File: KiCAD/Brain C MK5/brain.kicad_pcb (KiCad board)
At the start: 2 copper layers, 143 x 44.8 mm, 20 parts, among them J1 USB_B, J10 Conn_01x10, J11 Conn_01x10, J2 Conn_01x06, J3 Conn_01x10, J4 Conn_01x06, J5 Conn_01x06, J6 Conn_01x06, J7 Conn_01x04, J8 Conn_01x04, J9 Conn_01x10

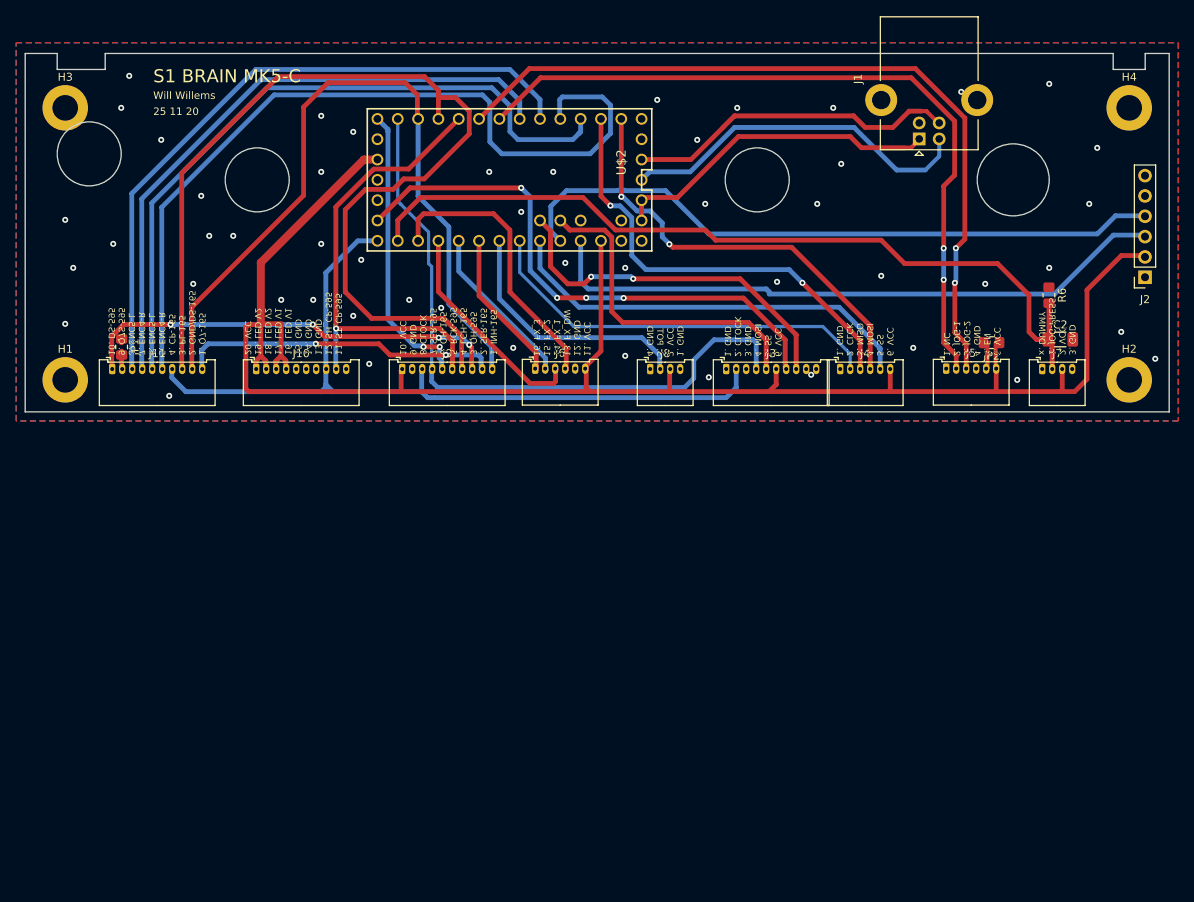
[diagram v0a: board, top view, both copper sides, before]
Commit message: add nect-gen KiCAD files
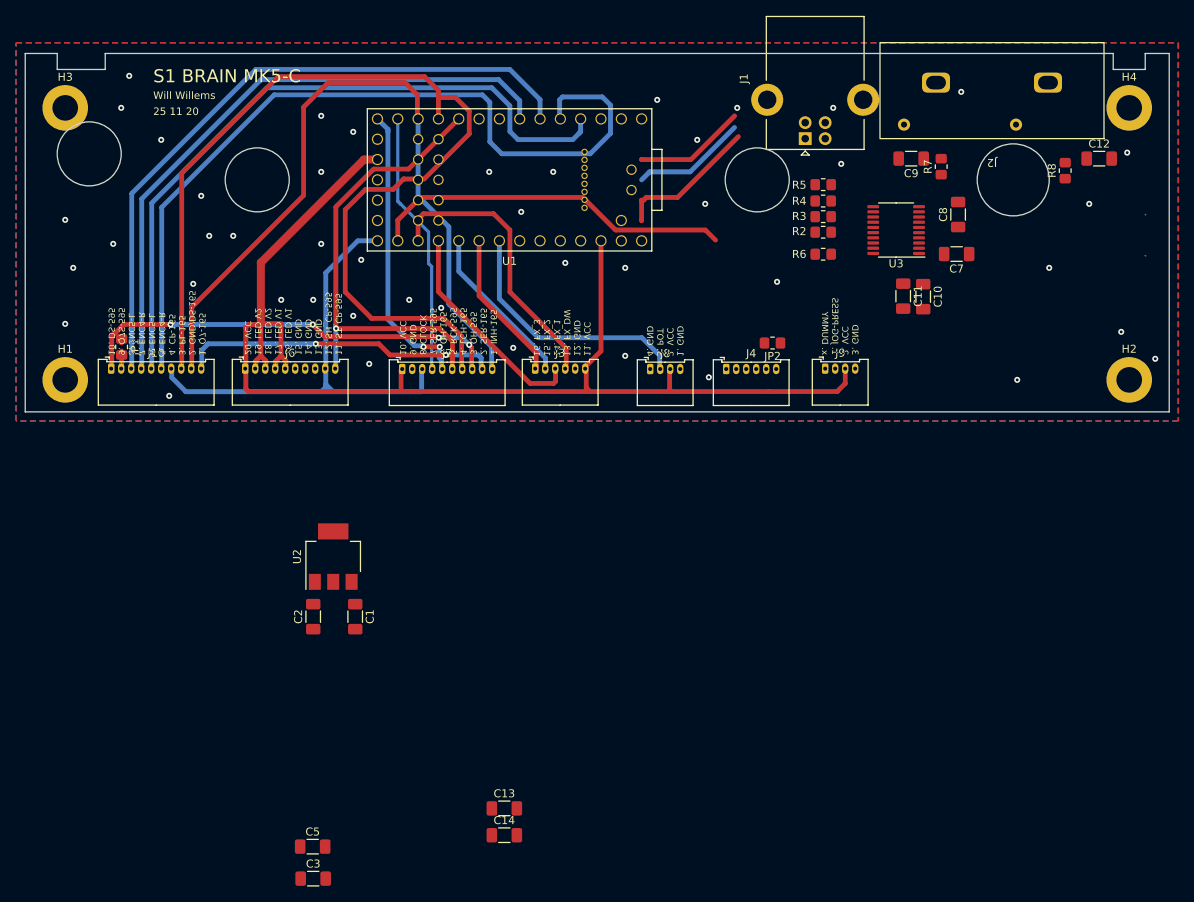
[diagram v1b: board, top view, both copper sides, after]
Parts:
- removed J11: Conn_01x10, Connector_Molex:Molex_PicoBlade_53048-1010_1x10_P1.25mm_Horizontal
- removed J5: Conn_01x06, Connector_Molex:Molex_PicoBlade_53048-0610_1x06_P1.25mm_Horizontal
- removed U$2: TEENSY_LC_ALL_PINS, brain:TEENSY_3.0-3.2&LC_ALL_PINS
- added C1: 100nF, Capacitor_SMD:C_1206_3216Metric_Pad1.33x1.80mm_HandSolder, F.Cu at (118.2, 153.0)
- added C10: 100nF, Capacitor_SMD:C_1206_3216Metric_Pad1.33x1.80mm_HandSolder, F.Cu at (189.2, 113.0)
- added C11: 10uF, Capacitor_SMD:C_1206_3216Metric_Pad1.33x1.80mm_HandSolder, F.Cu at (186.8, 112.9)
- added C12: 2.2nF, Capacitor_SMD:C_1206_3216Metric_Pad1.33x1.80mm_HandSolder, F.Cu at (211.2, 95.8)
- added C13: 100nF, Capacitor_SMD:C_1206_3216Metric_Pad1.33x1.80mm_HandSolder, F.Cu at (136.9, 177.0)
- added C14: 10uF, Capacitor_SMD:C_1206_3216Metric_Pad1.33x1.80mm_HandSolder, F.Cu at (136.9, 180.3)
- added C3: 100nF, Capacitor_SMD:C_1206_3216Metric_Pad1.33x1.80mm_HandSolder, F.Cu at (113.0, 185.8)
- added C5: 10uF, Capacitor_SMD:C_1206_3216Metric_Pad1.33x1.80mm_HandSolder, F.Cu at (112.9, 181.8)
- added C7: 2.2uF, Capacitor_SMD:C_1206_3216Metric_Pad1.33x1.80mm_HandSolder, F.Cu at (193.4, 107.7)
- added C8: 2.2uF, Capacitor_SMD:C_1206_3216Metric_Pad1.33x1.80mm_HandSolder, F.Cu at (193.6, 102.7)
- added C9: 2.2nF, Capacitor_SMD:C_1206_3216Metric_Pad1.33x1.80mm_HandSolder, F.Cu at (187.8, 95.8)
- added R2: 22, Resistor_SMD:R_0805_2012Metric_Pad1.20x1.40mm_HandSolder, F.Cu at (176.8, 105.0)
- added R3: 22, Resistor_SMD:R_0805_2012Metric_Pad1.20x1.40mm_HandSolder, F.Cu at (176.8, 103.0)
- added R4: 22, Resistor_SMD:R_0805_2012Metric_Pad1.20x1.40mm_HandSolder, F.Cu at (176.8, 101.0)
- added R5: 22, Resistor_SMD:R_0805_2012Metric_Pad1.20x1.40mm_HandSolder, F.Cu at (176.8, 99.0)
- added R7: 470, Resistor_SMD:R_0805_2012Metric_Pad1.20x1.40mm_HandSolder, F.Cu at (191.5, 96.8)
- added R8: 470, Resistor_SMD:R_0805_2012Metric_Pad1.20x1.40mm_HandSolder, F.Cu at (207.0, 97.2)
- added U1: Teensy4.0, Teensy:Teensy40_SMT, F.Cu at (137.5, 98.4)
- added U2: LD1117S33TR_SOT223, Package_TO_SOT_SMD:SOT-223-3_TabPin2, F.Cu at (115.5, 145.5)
- added U3: PCM5102, Package_SO:TSSOP-20_4.4x6.5mm_P0.65mm, F.Cu at (185.9, 104.7)
- C2: value 1u -> 10uF
- J2: value Conn_01x06 -> Conn_Coaxial_x2_Isolated; footprint Connector_PinSocket_2.54mm:PinSocket_1x06_P2.54mm_Vertical -> Audio:RCA_double
- J3: value Conn_01x10 -> Conn_01x06; footprint Connector_Molex:Molex_PicoBlade_53048-1010_1x10_P1.25mm_Horizontal -> Connector_Molex:Molex_PicoBlade_53048-0610_1x06_P1.25mm_Horizontal
- J6: value Conn_01x06 -> Conn_01x10; footprint Connector_Molex:Molex_PicoBlade_53048-0610_1x06_P1.25mm_Horizontal -> Connector_Molex:Molex_PicoBlade_53048-1010_1x10_P1.25mm_Horizontal
- J7: value Conn_01x04 -> Conn_01x10; footprint Connector_Molex:Molex_PicoBlade_53048-0410_1x04_P1.25mm_Horizontal -> Connector_Molex:Molex_PicoBlade_53048-1010_1x10_P1.25mm_Horizontal
- J9: value Conn_01x10 -> Conn_01x04; footprint Connector_Molex:Molex_PicoBlade_53048-1010_1x10_P1.25mm_Horizontal -> Connector_Molex:Molex_PicoBlade_53048-0410_1x04_P1.25mm_Horizontal
- R6: value 1M -> 0
- moved C2 99.6 mm to (113.0, 153.0), turned to 90 degrees
- moved J7 80.0 mm to (124.1, 122.0)
- moved J9 52.9 mm to (177.0, 122.0)
- moved J6 36.2 mm to (104.5, 122.0)
- moved J2 30.9 mm to (197.8, 86.2)
- moved R6 28.7 mm to (176.8, 107.7), turned to 0 degrees
- moved JP2 27.4 mm to (170.4, 118.8)
- moved J3 23.9 mm to (140.8, 122.0)
- moved J10 18.1 mm to (87.8, 122.0)
- moved J1 14.3 mm to (174.5, 93.2)
- moved J4 14.2 mm to (164.6, 122.0)
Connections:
- C2 pad 1: /JOG-PRESS-IR -> VDDA
- J1 pad 1: Net-(U$2-PadVIN_PAD) -> unconnected-(J1-VBUS-Pad1)
- J1 pad 2: Net-(U$2-PadD-) -> unconnected-(J1-D--Pad2)
- J1 pad 3: Net-(U$2-PadD+) -> unconnected-(J1-D+-Pad3)
- J10 pad 1: +3.3V -> /595-BRIDGE
- J10 pad 10: /595-LATCH -> /165-BRIDGE
- J10 pad 2: +3.3V -> /595-OUT-MAIN
- J10 pad 3: +3.3V -> /ENCR1
- J10 pad 4: +3.3V -> /ENCR2
- J10 pad 5: +3.3V -> /ENCL1
- J10 pad 6: GND -> /ENCL2
- J10 pad 7: GND -> /CLOCK
- J10 pad 8: GND -> /165-LATCH
- J10 pad 9: /CLOCK -> /CE-595-165
- J2 pad 1: GND -> /PCM5102/AUDIO_OUT_R
- J2 pad 2: +3.3V -> GND
- J2 pad 3: /SDA-EXT -> /PCM5102/AUDIO_OUT_L
- J2 pad 4: /SCL-EXT -> GND
- J3 pad 1: GND -> /POT4
- J3 pad 2: /CLOCK -> /POT3
- J3 pad 3: GND -> /POT2
- J3 pad 4: /MOSI -> /POT1
- J3 pad 5: /SS-SCREEN -> GND
- J4 pad 1: GND -> unconnected-(J4-Pin_1-Pad1)
- J4 pad 2: /CLOCK-EXT -> /JOG-MOVE1
- J4 pad 3: /MISO-EXT -> /JOG-MOVE2
- J4 pad 4: /MOSI-EXT -> GND
- J4 pad 5: /SS-EXT -> Net-(J4-Pin_5)
- J6 pad 1: /POT4 -> +3.3V
- J6 pad 2: /POT3 -> +3.3V
- J6 pad 3: /POT2 -> +3.3V
- J6 pad 4: /POT1 -> +3.3V
- J6 pad 5: GND -> +3.3V
- J6 pad 6: +3.3V -> GND
- J7 pad 1: unconnected-(J7-Pad1) -> +3.3V
- J7 pad 2: /JOG-PRESS-IR -> GND
- J7 pad 3: +3.3V -> /CLOCK
- J7 pad 4: GND -> unconnected-(J7-Pin_4-Pad4)
- J9 pad 1: +3.3V -> unconnected-(J9-Pin_1-Pad1)
- J9 pad 2: GND -> /JOG-PRESS-IR
- J9 pad 3: /CLOCK -> +3.3V
- J9 pad 4: unconnected-(J9-Pad4) -> GND
- JP2 pad 2: Net-(JP2-Pad2) -> Net-(J4-Pin_5)
- R6 pad 1: /JOG-PRESS-IR -> GND
- R6 pad 2: GND -> Net-(U3-FMT)
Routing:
- net /JOG-MOVE2: track 98.8 -> 0.32 mm, vias 2 -> 0
- net /JOG-MOVE1: track 93.9 -> 0.26 mm, vias 2 -> 0
- net /MOSI: track 83.9 -> 0.00 mm
- net /SCL-EXT: track 83.5 -> 0.00 mm
- net /SDA-EXT: track 79.7 -> 0.00 mm
- net /DC-SCREEN: track 69.7 -> 0.00 mm, vias 4 -> 0
- net /CE-595-165: track 93.5 -> 153.4 mm, vias 0 -> 1
- net /595-LATCH: track 59.9 -> 0.00 mm, vias 1 -> 0
- net /JOG-PRESS-IR: track 103.5 -> 45.9 mm
- net /MISO-EXT: track 56.3 -> 0.28 mm, vias 2 -> 0
- net GND: track 0.00 -> 54.8 mm, vias 48 -> 47
- net /595-BRIDGE: track 54.7 -> 0.00 mm, vias 4 -> 0
- net /MOSI-EXT: track 54.3 -> 0.19 mm, vias 2 -> 0
- net /SS-EXT: track 52.9 -> 0.00 mm
- net /CLOCK-EXT: track 51.6 -> 0.00 mm
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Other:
- board text removed: "6. VCC 5. EN 4. GND 3. JOG-2 2. JOG-1 1. NC"
- board text removed: "6. VCC 5. SS 4. MOSI 3. GND 2. CLOCK 1. GND"
- board text removed: "6. VCC 5. SS 4. MOSI 3. MISO 2. CLCK 1. GND"
